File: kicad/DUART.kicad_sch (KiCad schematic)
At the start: 6 parts

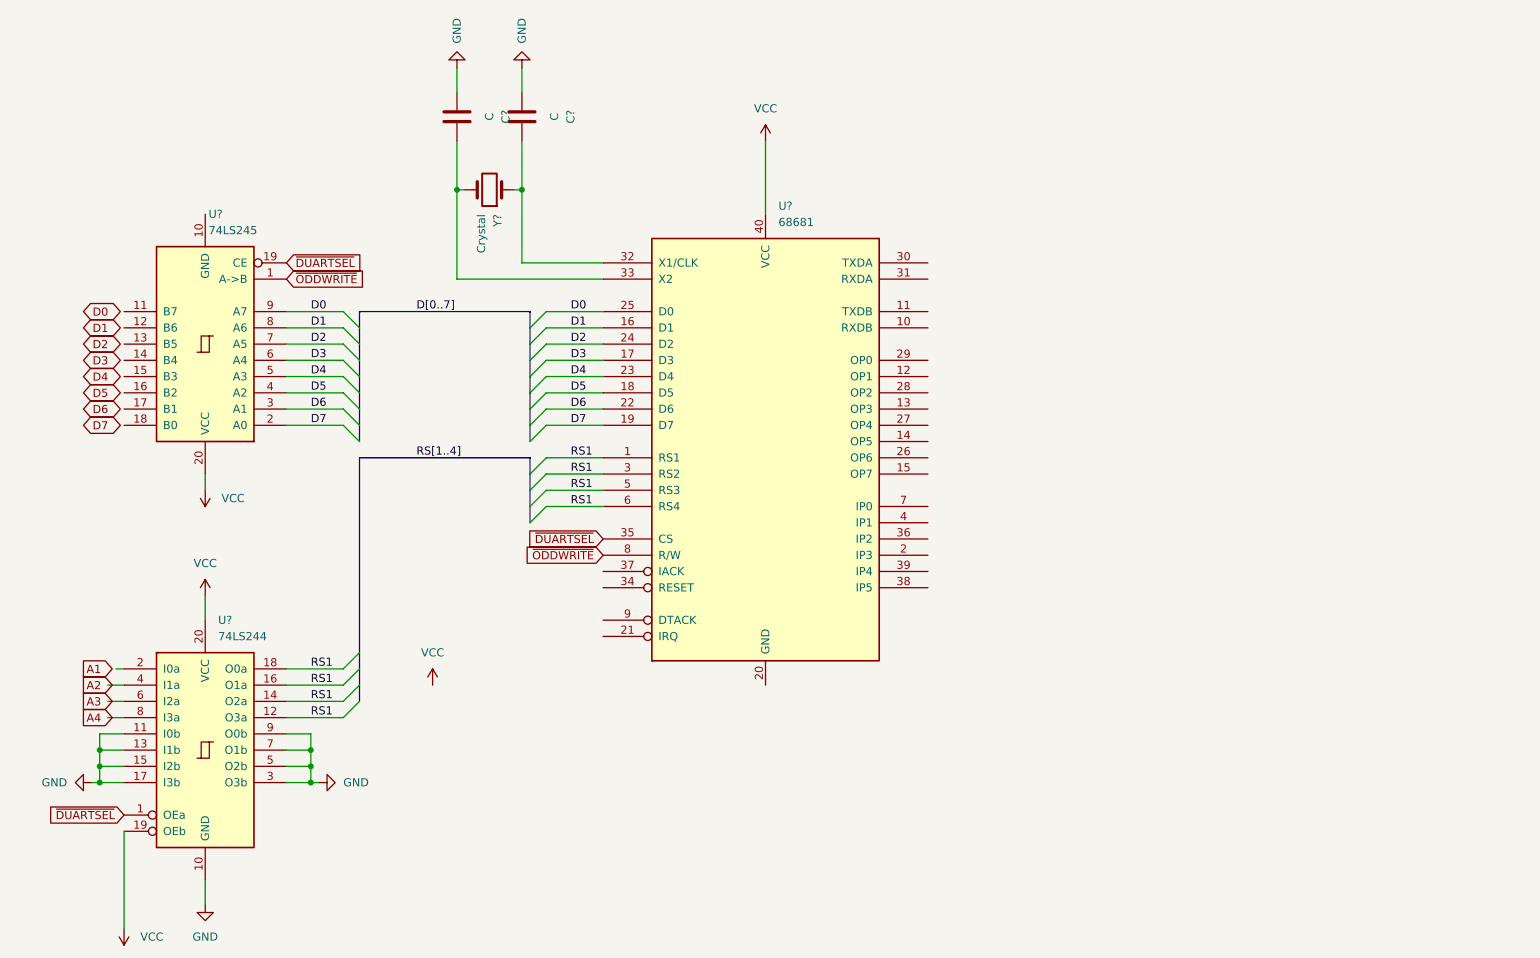
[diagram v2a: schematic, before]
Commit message: started with pcb
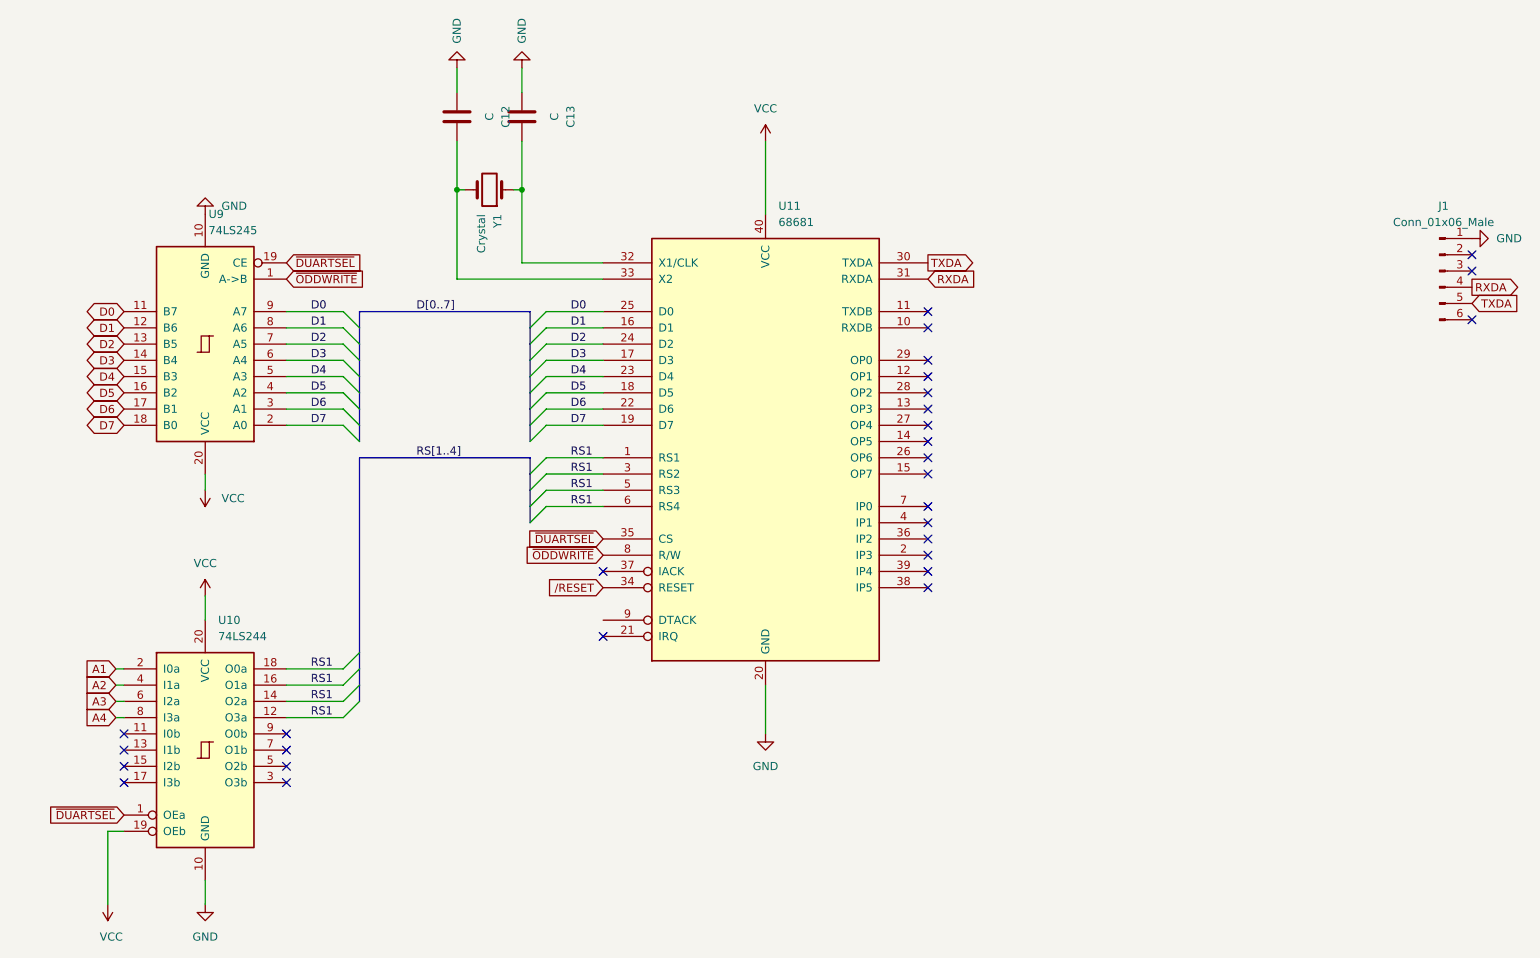
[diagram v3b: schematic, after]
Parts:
- added J1: Conn_01x06_Male, Connector_PinHeader_2.54mm:PinHeader_1x06_P2.54mm_Vertical, symbol Connector:Conn_01x06_Male
- C12, C13: renamed from C?; footprint (none) -> Capacitor_THT:CP_Radial_D8.0mm_P5.00mm
- U10, U9: renamed from U?; footprint (none) -> Package_DIP:DIP-20_W7.62mm_Socket
- U11: renamed from U?; footprint (none) -> Package_DIP:DIP-40_W15.24mm_Socket
- Y1: renamed from Y?; footprint (none) -> Crystal:Crystal_HC18-U_Vertical
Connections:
- net A1: now also U10.2 (I0a)
- net A2: now also U10.4 (I1a)
- net A3: now also U10.6 (I2a)
- net A4: now also U10.8 (I3a)
- net D0: now also U9.11 (B7)
- net D1: now also U9.12 (B6)
- net D2: now also U9.13 (B5)
- net D3: now also U9.14 (B4)
- net D4: now also U9.15 (B3)
- net D5: now also U9.16 (B2)
- net D6: now also U9.17 (B1)
- net D7: now also U9.18 (B0)
- net GND: now also U11.20 (GND), U9.10 (GND), J1.1 (Pin_1); no longer U10.11 (I0b), U10.13 (I1b), U10.15 (I2b), U10.17 (I3b), U10.3 (O3b), U10.5 (O2b), U10.7 (O1b), U10.9 (O0b)
- net TXDA: now reaches U11.30 (TXDA)
- net TXDA: now also J1.5 (Pin_5)
- net RXDA: now reaches U11.31 (RXDA)
- net RXDA: now also J1.4 (Pin_4)
- net /RESET: now reaches U11.34 (RESET)
- no-connect marks 0 -> 29
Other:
- title: (none) -> Mats Brorson 68010 SBC DUART 68681

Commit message: Update footprint
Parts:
- C12, C13: footprint Capacitor_THT:CP_Radial_D8.0mm_P5.00mm -> Capacitor_THT:CP_Radial_D5.0mm_P2.50mm
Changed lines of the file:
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@@
     (property "Reference" "C12" (id 0) (at 101.6 33.02 90))
     (property "Value" "C" (id 1) (at 99.06 33.02 90))
-    (property "Footprint" "Capacitor_THT:CP_Radial_D8.0mm_P5.00mm" (id 2) (at 94.9452 36.83 0)
+    (property "Footprint" "Capacitor_THT:CP_Radial_D5.0mm_P2.50mm" (id 2) (at 94.9452 36.83 0)
       (effects (font (size 1.27 1.27)) hide)
     )
@@
     (property "Reference" "C13" (id 0) (at 111.76 33.02 90))
     (property "Value" "C" (id 1) (at 109.22 33.02 90))
-    (property "Footprint" "Capacitor_THT:CP_Radial_D8.0mm_P5.00mm" (id 2) (at 105.1052 36.83 0)
-      (effects (font (size 1.27 1.27)) hide)
-    )
+    (property "Footprint" "Capacitor_THT:CP_Radial_D5.0mm_P2.50mm" (id 2) (at 105.1052 36.83 0)
+      (effects (font (size 1.27 1.27)) hide)
+    )

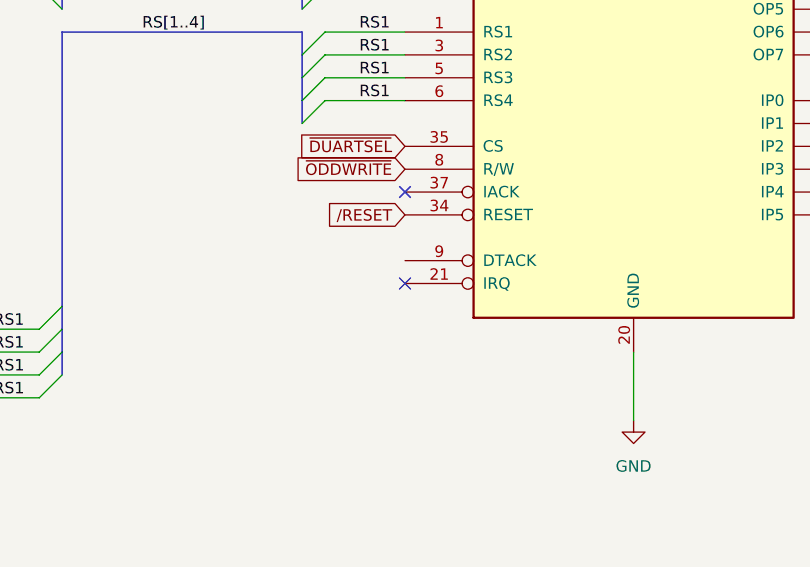
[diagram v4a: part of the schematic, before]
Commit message: cleanup
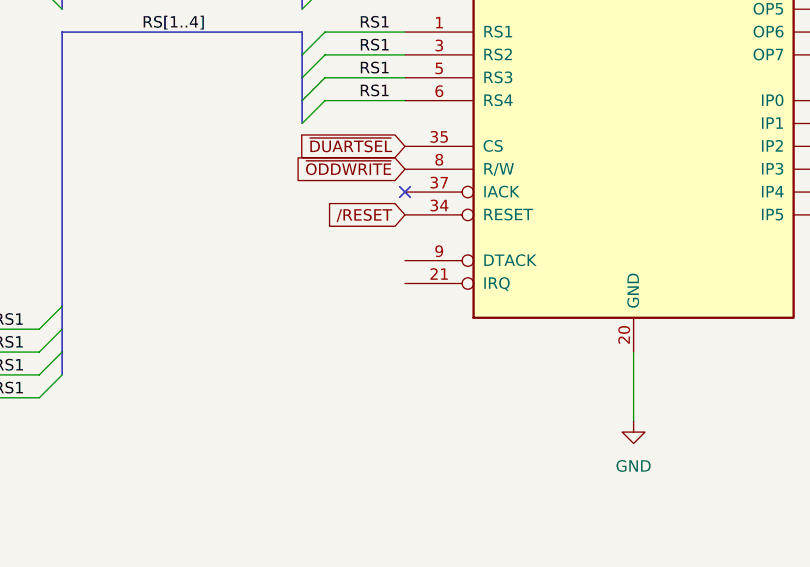
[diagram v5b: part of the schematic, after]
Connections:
- no-connect marks 29 -> 28
